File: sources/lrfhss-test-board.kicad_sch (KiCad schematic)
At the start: 19 parts, among them J1 USB-C, J2 532610271, J3 532610271, J4 532610471, U1 LoRa126XF30, U2 AMS1117-3.3

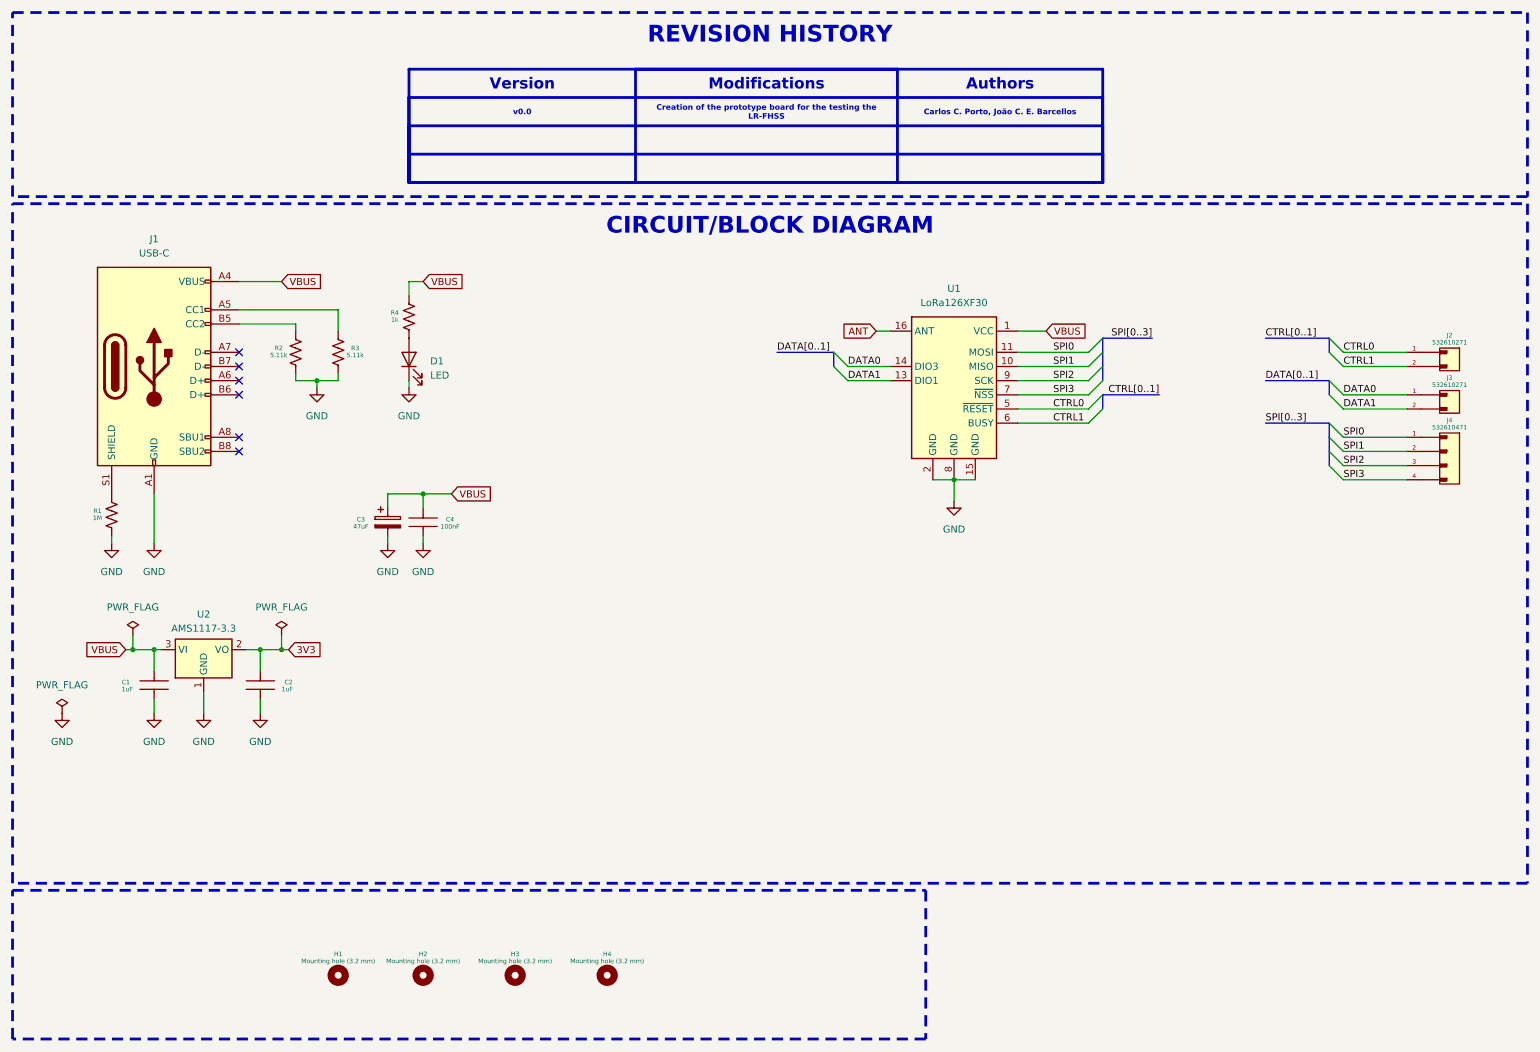
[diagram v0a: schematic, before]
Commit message: feat: improve schematic and layout
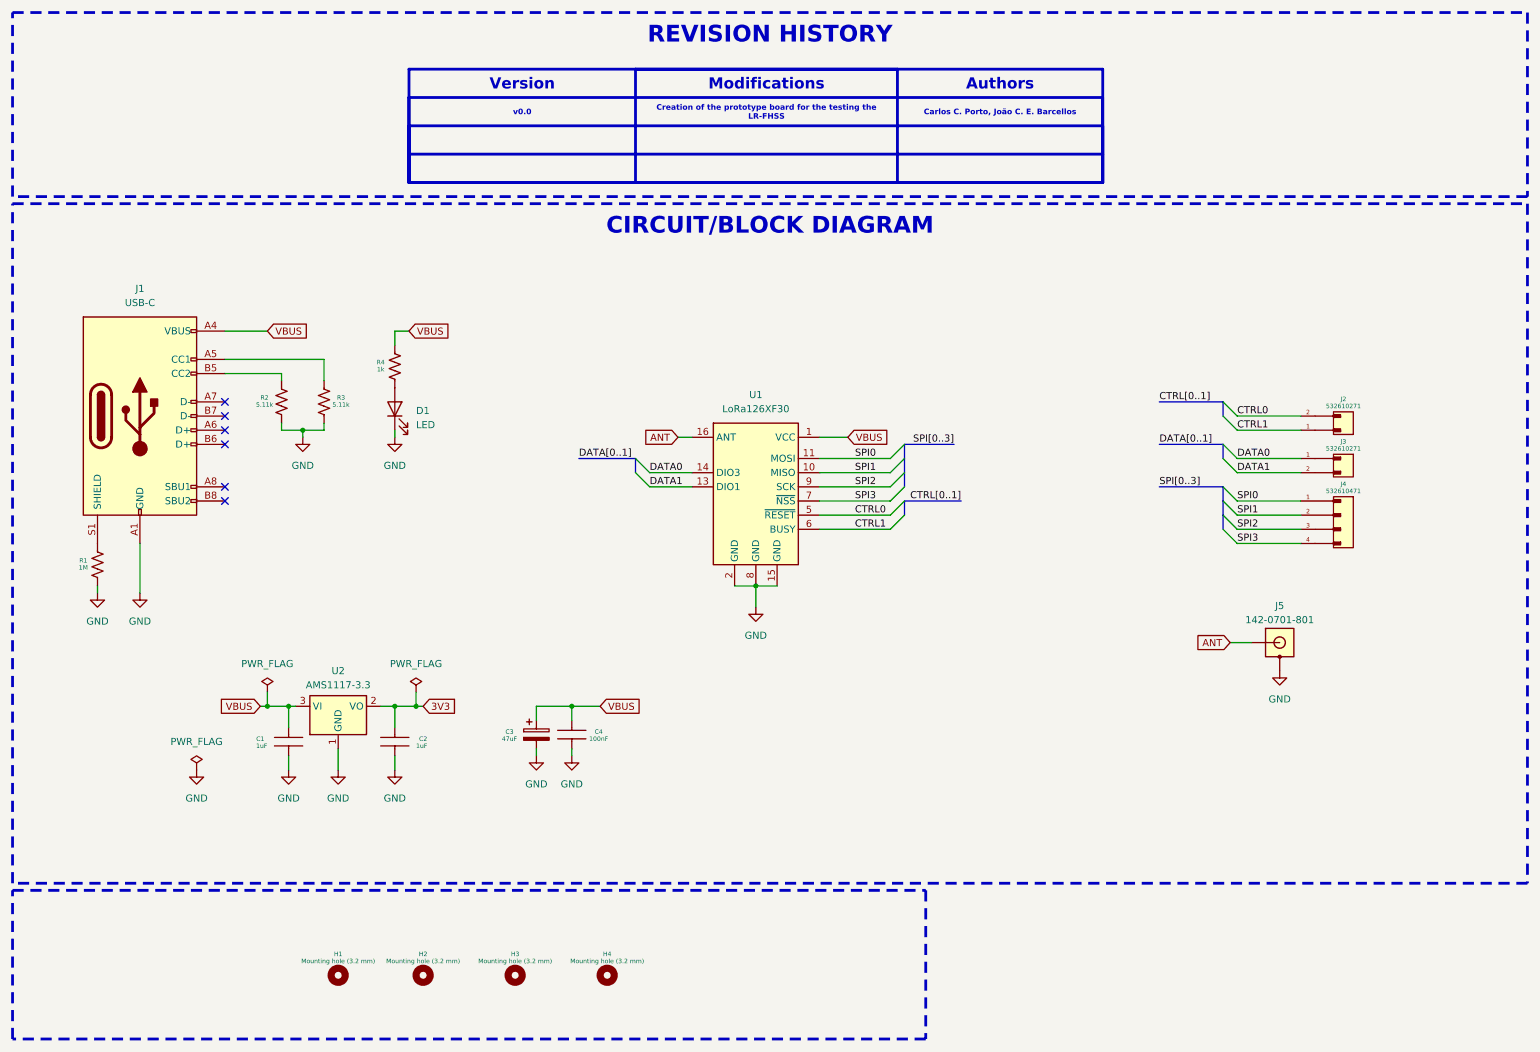
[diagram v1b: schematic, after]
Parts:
- added J5: 142-0701-801, footprints:142-0701-801, symbol connectors:142-0701-801
- D1: footprint (none) -> LED_SMD:LED_0603_1608Metric
- J1: footprint footprinst:GENERIC-USB-C.step -> footprints:GENERIC-USB-C
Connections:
- net ANT: now also J5.1
- net CTRL0: now also J2.2; no longer J2.1
- net CTRL1: now also J2.1; no longer J2.2
- net GND: now also J5.S1, J5.S2, J5.S3, J5.S4
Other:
- moved on the sheet: C1, C2, C3, C4, D1, J1, J2, J3, J4, R1, R2, R3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
